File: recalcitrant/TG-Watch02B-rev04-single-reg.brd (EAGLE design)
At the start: 36.8 x 40.6 mm, 66 parts, among them IC3 W25Q128JVSIQ TR, J1 USB-C-CON-TG_MOD-2295018-2.0, J2 DISP_1.54_LCMTF15423A-C_LCD+C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, J3 CON-BAT-TG-MEZ_FEMALE, Q3 DMG2305, U2 MICROBUILDER_LSM6DSOX, U3 VREG-TPS63036, U4 FAN5331SX, U5 MCP73831/OT, U6 LC709203F, U8 UNDERVOLT-TPS3702CX3

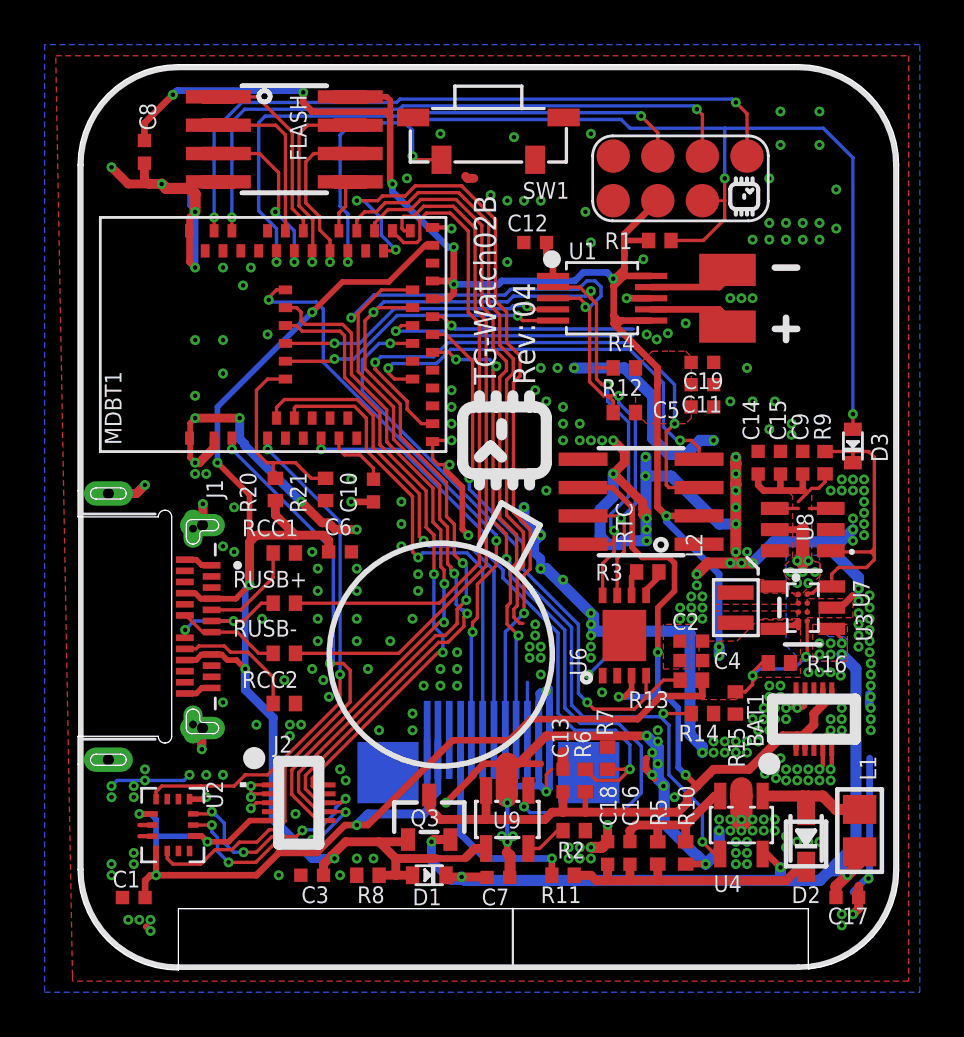
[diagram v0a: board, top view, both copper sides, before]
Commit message: pre-order
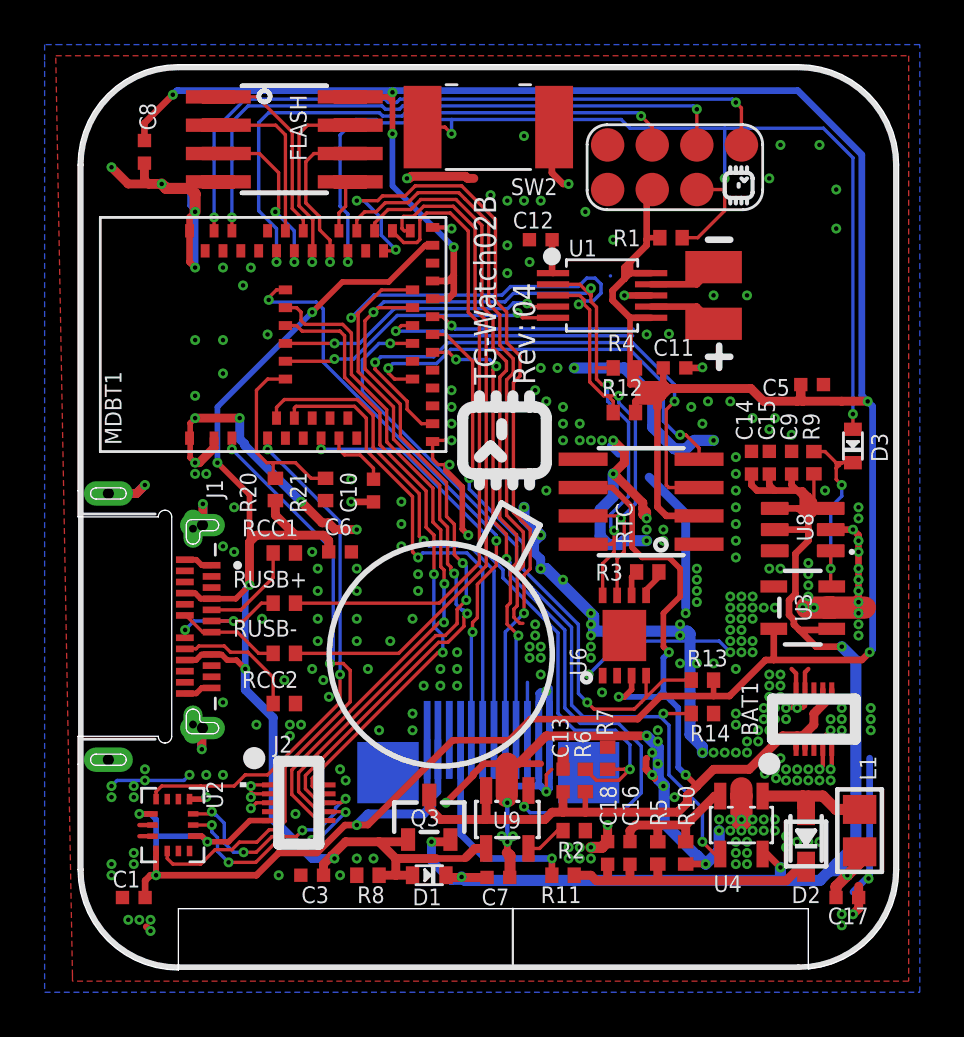
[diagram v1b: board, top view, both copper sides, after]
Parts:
- removed C19, C2, C4: 10uf, 0TG-Lib v01.5:MICROBUILDER__0402_NODIMS
- removed L2: 1uH - HMLQ20161B-1R0MDR, FPV_Static-Lib_v1.1:NONSTANDARD_INDUCTOR_5
- removed R15: 59k, 0TG-Lib v01.5:TG_0402
- removed R16: 330k, 0TG-Lib v01.5:TG_0402
- removed SW1: (no value), 0TG-Lib v01.5:MICROBUILDER_SPST_TACTILE_RA_NO_ALIGN
- removed U7: (no value), 0TG-Lib v01.4:SOT23-5
- added SW2: (no value), 0TG-Lib v01.5:BTN_CK_KSS
- D3: value BAS16XV2T1G -> (none)
- U3: value VREG-TPS63036 -> (none); device 0TG-Lib v01.5:TPS63036YFGR_BGA8N40P4X2_NOSILK -> 0TG-Lib v01.4:SOT23-5
- moved C5 5.02 mm to (32.9, 26.3)
- moved C11 1.46 mm to (26.8, 27.0)
- moved HEDR2 0.64 mm to (28.5, 30.2)
- moved U$3 0.56 mm to (25.8, 36.0)
- moved R1 0.52 mm to (26.6, 32.8)
- moved C15 0.50 mm to (31.0, 22.8)
- moved C9 0.50 mm to (32.0, 22.8)
- moved R13 0.50 mm to (28.0, 13.0)
- moved R9 0.50 mm to (33.0, 22.8)
- moved C14 0.30 mm to (30.2, 22.8)
- moved C12 0.28 mm to (20.8, 32.8)
- moved U1 0.12 mm to (23.5, 30.2)
- turned U3 to 90 degrees
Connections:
- removed net L1: L2.1, U3.B1
- removed net L2: L2.2, U3.C1
- removed net SENSE: R15.2, R16.2, U3.D2
- net 3V3: now also U3.5; no longer C19.2, C2.2, C4.2, R16.1, U3.D1, U7.5
- net GND: now also SW2.P$1, U3.2; no longer C19.1, C2.1, C4.1, R15.1, SW1.1, U3.B2, U3.C2, U7.2
- net RESET: now also SW2.P$2; no longer SW1.2
- net SYS_EN: now also U3.3; no longer U3.A2, U7.3
- net VSORS: now also U3.1; no longer U3.A1, U7.1
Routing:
- net 3V3: track 118.3 -> 176.9 mm, vias 13 -> 10
- net VSORS: track 51.3 -> 63.9 mm, vias 17 -> 5
- net SENSE: track 6.71 -> 0.00 mm, vias 2 -> 0
- net SYS_EN: track 13.8 -> 9.16 mm, vias 0 -> 2
- net GND: track 177.8 -> 181.0 mm, vias 331 -> 323
- net RESET: track 53.9 -> 52.6 mm
- net HAPTIC-: track 3.98 -> 3.13 mm
- net D12_BAT_INT: track 25.6 -> 26.1 mm
- removed copper zone on layer 1, net 3V3
- removed copper zone on layer 1, net L1
- removed copper zone on layer 1, net L2
- removed copper zone on layer 1, net VSORS
- removed copper zone on layer 16, net VSORS
